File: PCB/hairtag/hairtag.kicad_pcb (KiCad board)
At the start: 2 copper layers, 24 x 24 mm, 27 parts, among them J1 Flash, J2 BAT, U1 ESP32-C3FH4, X1 XL2EL89CPI-111YLC-40M

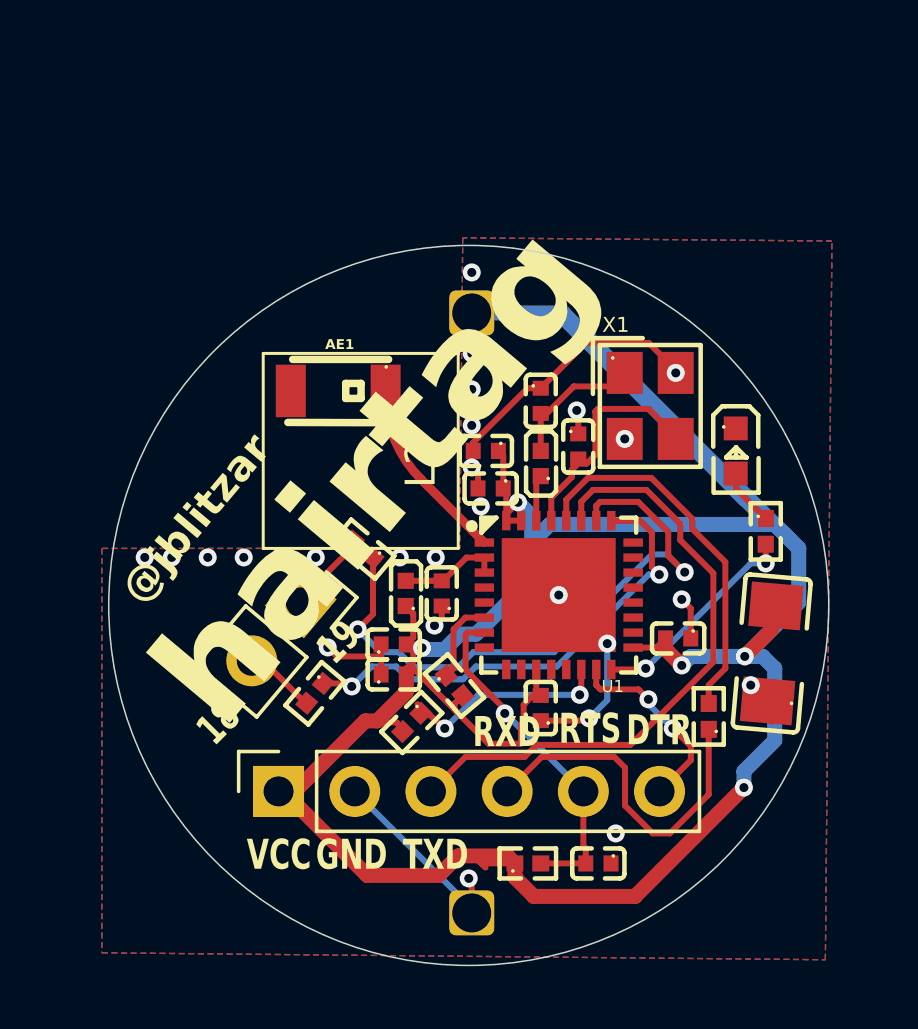
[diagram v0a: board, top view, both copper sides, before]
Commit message: OMG OMG OMG
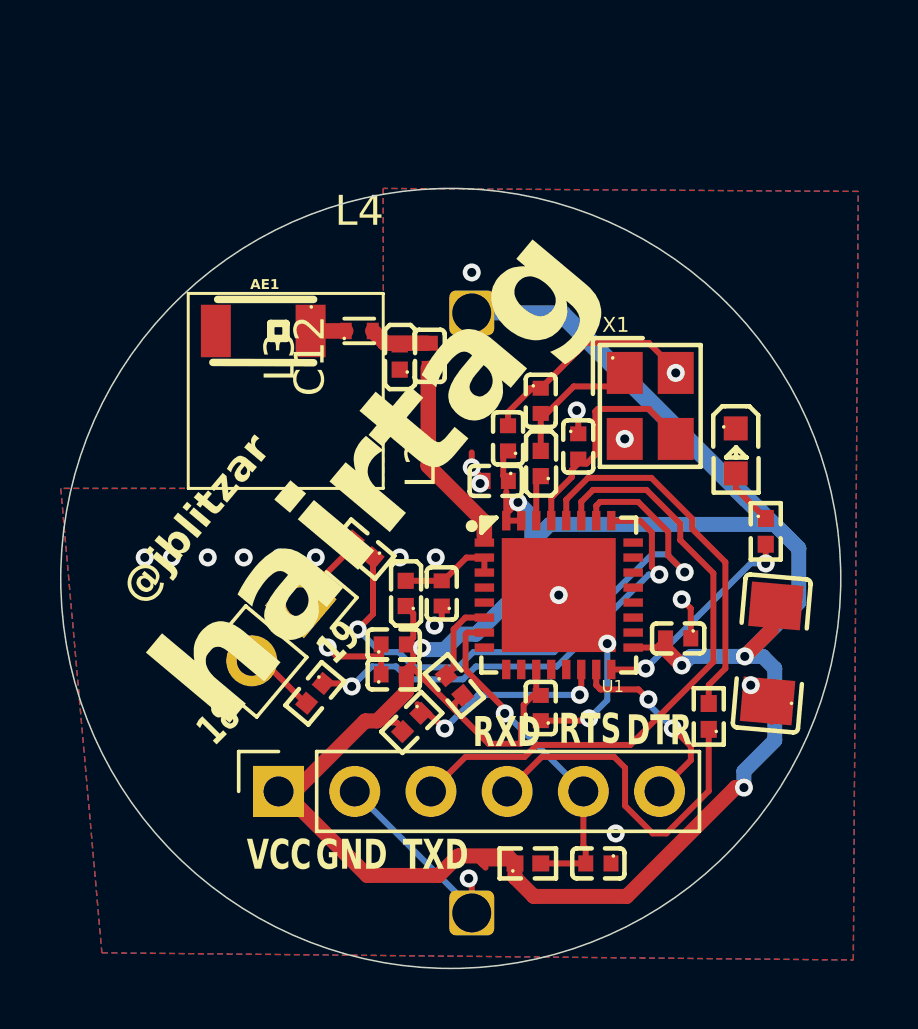
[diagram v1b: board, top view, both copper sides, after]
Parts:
- added C12: 1pF, easyeda2kicad:C0402, F.Cu at (53.8, 47.1)
- added L3: 2.7nH, easyeda2kicad:L0402, F.Cu at (52.8, 47.1)
- added L4: 3.9nH, easyeda2kicad:IND-SMD_L1.0-W0.5-2, F.Cu at (51.5, 46.2)
- moved AE1 3.20 mm to (48.2, 46.2)
- moved C5 0.85 mm to (56.4, 49.8), turned to 90 degrees
- moved C6 0.30 mm to (56.0, 51.2)
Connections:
- AE1 pad 1: /LNA_IN -> Net-(AE1-ANT)
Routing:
- net Net-(C12-Pad2): track 0.00 -> 1.97 mm
- net Net-(AE1-ANT): track 0.00 -> 1.17 mm
- net GND: track 27.6 -> 26.4 mm, vias 26 -> 23
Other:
- board size 24 x 24 mm -> 26 x 26 mm
